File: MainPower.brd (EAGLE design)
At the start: 160 x 100 mm, 10 parts, among them IC1 RV-3029-C2

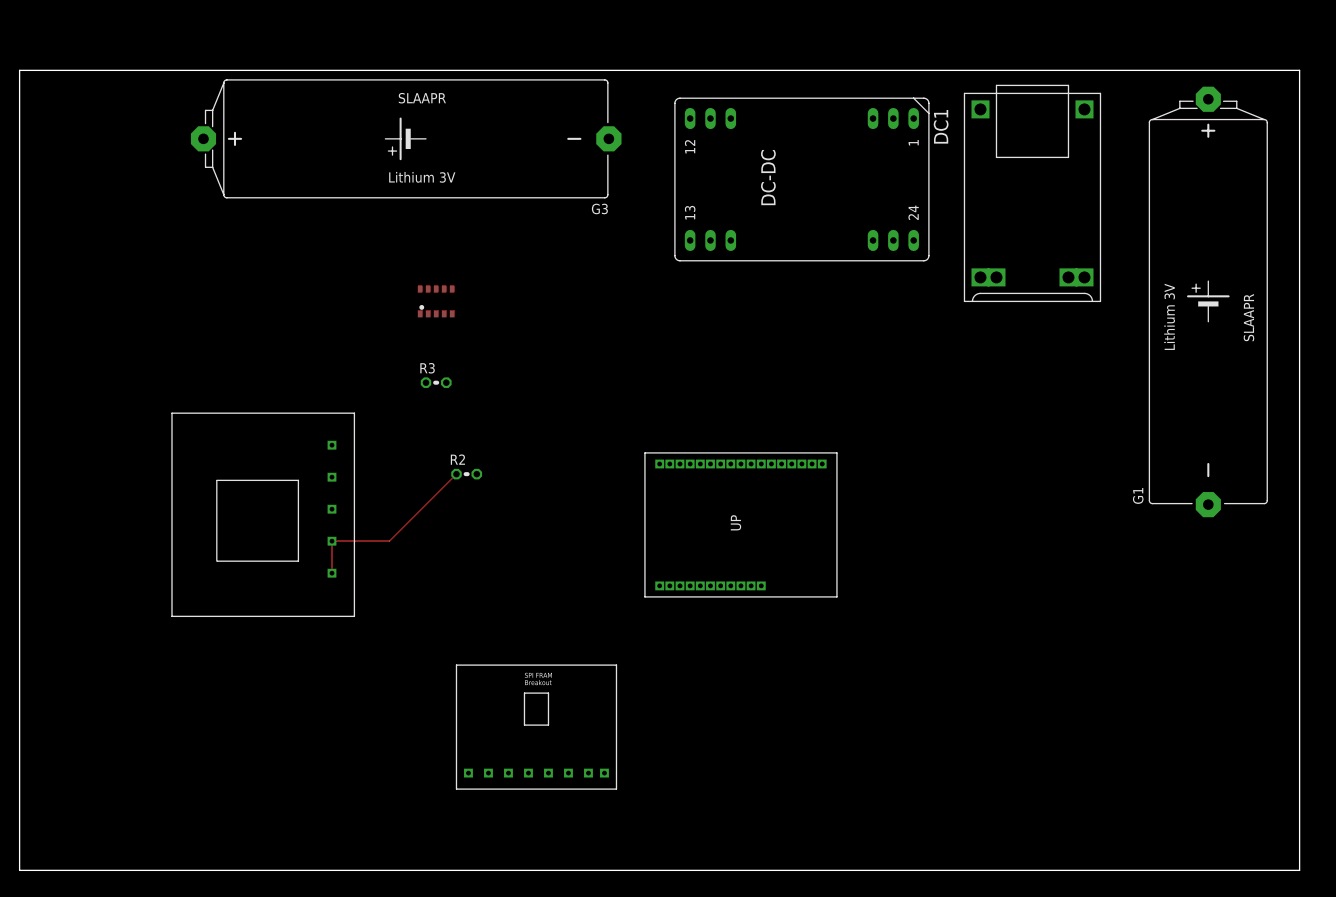
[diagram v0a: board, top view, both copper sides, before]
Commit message: Add files via upload
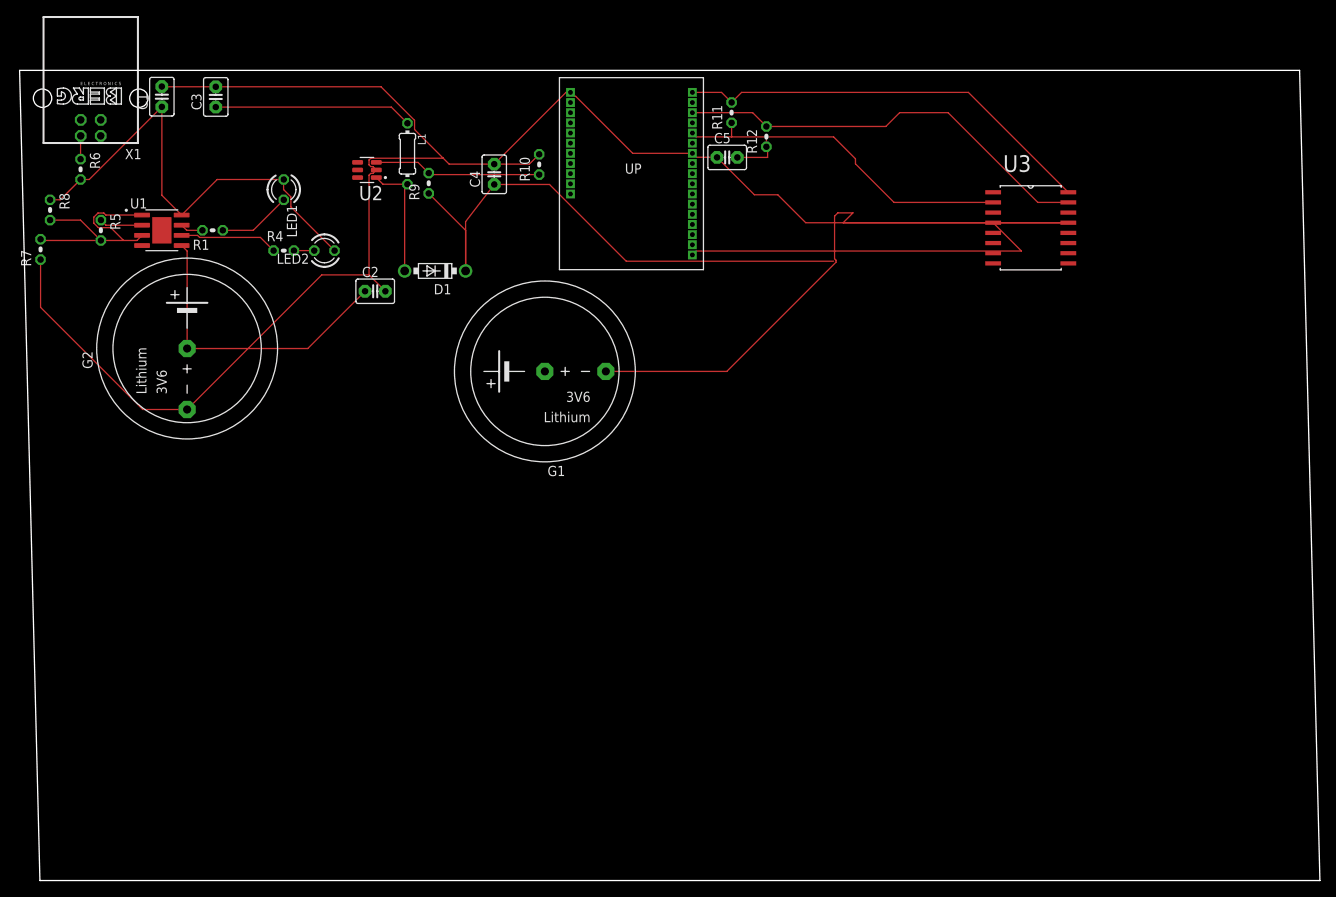
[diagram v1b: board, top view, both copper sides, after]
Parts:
- removed DC1: (no value), dc-dc-converter:CMK
- removed G3: SL-160AA/PR, battery:SL-160AA/PR
- removed IC1: RV-3029-C2, crystal:SON-10
- removed R2, R3: 10k, rcl:0204V
- removed U$1: TP4056, TP4056:TP4056_FTP
- removed U$3: FRAM, fram:FRAMFT
- removed U$4: SCD40, SCD40:SCD-40FT
- added C1, C2, C3, C4, C5: 10uF, capacitor-wima:C2.5-3
- added D1: 1N5819-B, diode:DO41-7.6
- added G2: SL-340/P3.6V, battery:SL-340/P3.6V
- added L1: (no value), rcl:0204/7
- added LED1: TLLR4400, led:LED3MM
- added LED2: TLLG4400, led:LED3MM
- added R1, R10, R4, R5, R6, R7, R8, R9: 1k, rcl:0204V
- added R11, R12: 10k, rcl:0204V
- added U1: TP4056, TP4056:SOP127P600X175-9N
- added U2: MT3608, MT3608:SOT95P280X145-6N
- added U3: DS3231S, DS3231S:SOIC127P1032X265-16N
- added X1: (no value), con-berg:PN61729
- G1: value SL-160AA/PR -> SL-340/P3.6V; device battery:SL-160AA/PR -> battery:SL-340/P3.6V
- moved G1 83.4 mm to (65.7, 62.4), turned to 180 degrees
- moved U$2 39.6 mm to (80.3, 84.5), turned to 180 degrees
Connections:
- removed net IN+: U$1.6
- removed net N$1: G3.+, IC1.8
- new net CLK_RST: U$2.1, U3.4
- new net N$10: R1.2, U1.7
- new net N$11: C2.1, C3.1, G2.+, L1.1, U1.5, U2.4, U2.5
- new net N$12: R10.1, R9.2, U2.3
- new net N$8: LED2.K, R4.2
- new net N$9: LED1.K, R1.1
- new net USB: C1.1, LED1.A, LED2.A, R6.1, R6.2, R8.1, U1.4, U1.8, X1.1
- net 5V: now also C4.1, C5.2, D1.C, R11.1, R12.1, R9.1, U3.2; no longer DC1.14, IC1.1, R2.1, R3.1, U$4.1, U$4.2
- net GND: now also C1.2, C2.2, C3.2, C4.2, C5.1, G1.-, G2.-, R10.2, R5.2, R7.1, R7.2, R8.2, U1.1, U1.3, U2.2, U3.13; no longer DC1.15, G3.-, IC1.6, U$3.2, U$4.3
- net N$2: now also D1.A, L1.2, U2.1; no longer G1.+, U$1.2
- net N$3: now also R4.1, U1.6; no longer G1.-, U$1.3
- net N$4: now also G1.+, U3.14; no longer DC1.13, U$1.4
- net N$5: now also R5.1, U1.2; no longer DC1.24, U$1.1
- net SCL: now also R11.2, U3.16; no longer IC1.4, R3.2, U$4.4
- net SDA: now also R12.2, U3.15; no longer IC1.5, R2.2, U$4.5
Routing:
- net GND: track 0.00 -> 326.7 mm
- net 5V: track 23.0 -> 119.7 mm
- net N$11: track 0.00 -> 63.2 mm
- net USB: track 0.00 -> 62.4 mm
- net SCL: track 0.00 -> 53.2 mm
- net SDA: track 0.00 -> 53.1 mm
- net CLK_RST: track 0.00 -> 46.3 mm
- net N$12: track 0.00 -> 21.0 mm
- net N$2: track 0.00 -> 15.4 mm
- net N$3: track 0.00 -> 12.3 mm
- net N$9: track 0.00 -> 9.20 mm
- net N$5: track 0.00 -> 5.41 mm
- net N$10: track 0.00 -> 2.87 mm
- net N$8: track 0.00 -> 2.54 mm
- net N$4: track 0.00 -> 0.50 mm
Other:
- board size 160 x 100 mm -> 162.5 x 101.3 mm
